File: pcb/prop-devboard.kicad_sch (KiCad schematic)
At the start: 11 parts, among them SW1 SW_Push, U1 STM32G0B1CBT6, Y1 32.768 KHz, 10ppm, 12.5pf, Y2 8 MHz, 10ppm, 10pf

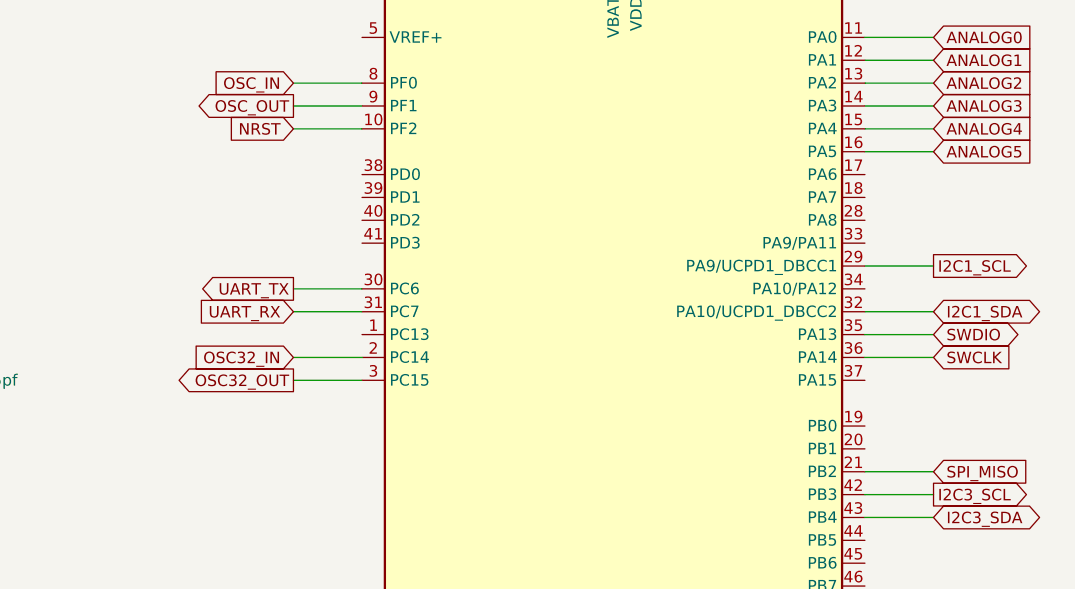
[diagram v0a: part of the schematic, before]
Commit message: Mostly finished PCB layout
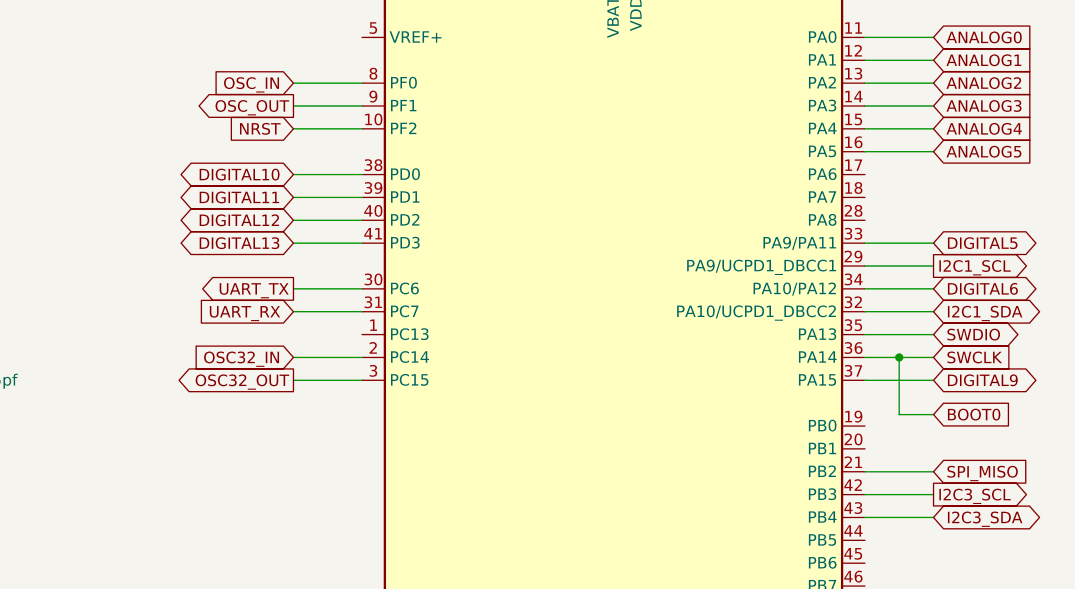
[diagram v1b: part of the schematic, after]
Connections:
- net DIGITAL5: now reaches U1.33 (PA9/PA11)
- net DIGITAL6: now reaches U1.34 (PA10/PA12)
- net DIGITAL9: now reaches U1.37 (PA15)
- net DIGITAL10: now reaches U1.38 (PD0)
- net DIGITAL11: now reaches U1.39 (PD1)
- net DIGITAL12: now reaches U1.40 (PD2)
- net DIGITAL13: now reaches U1.41 (PD3)
- net SWCLK renamed BOOT0
